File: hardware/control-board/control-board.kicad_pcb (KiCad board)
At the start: 2 copper layers, 39 x 110 mm, 44 parts, among them J10 Conn_01x09_Socket, J11 Conn_01x09_Socket, J12 Conn_01x12_Pin, J9 Conn_01x13_Socket

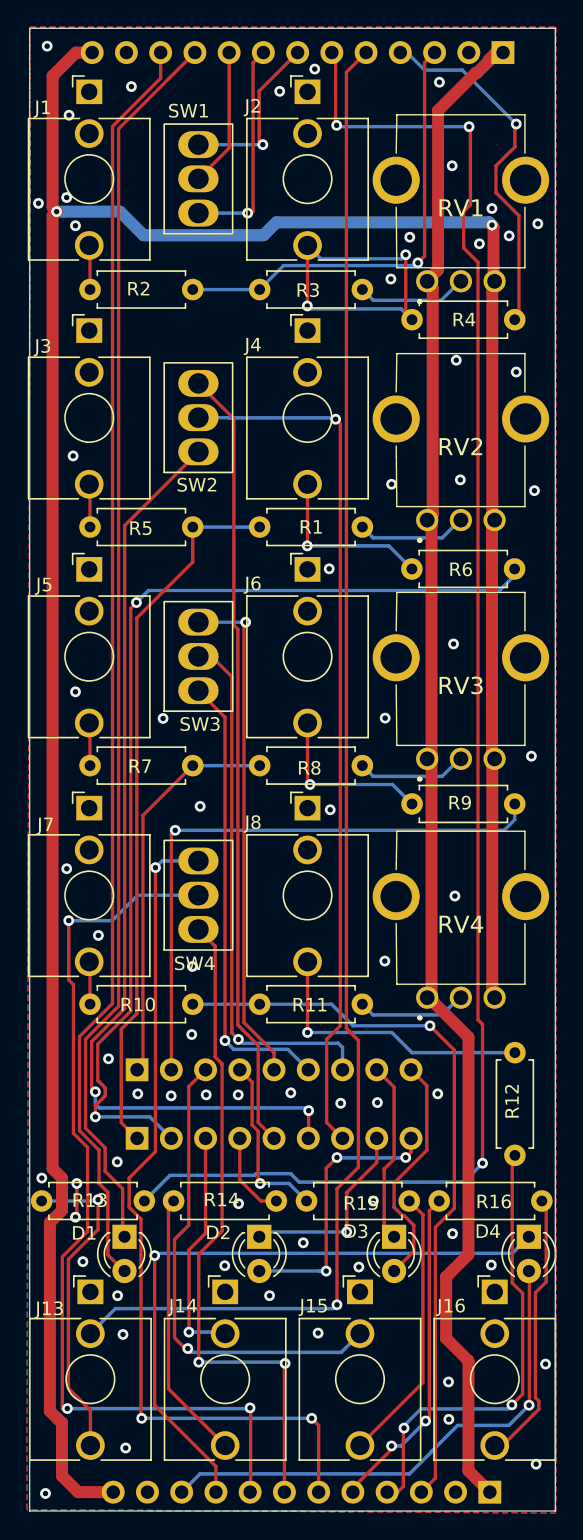
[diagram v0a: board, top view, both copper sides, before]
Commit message: wip - first pass done
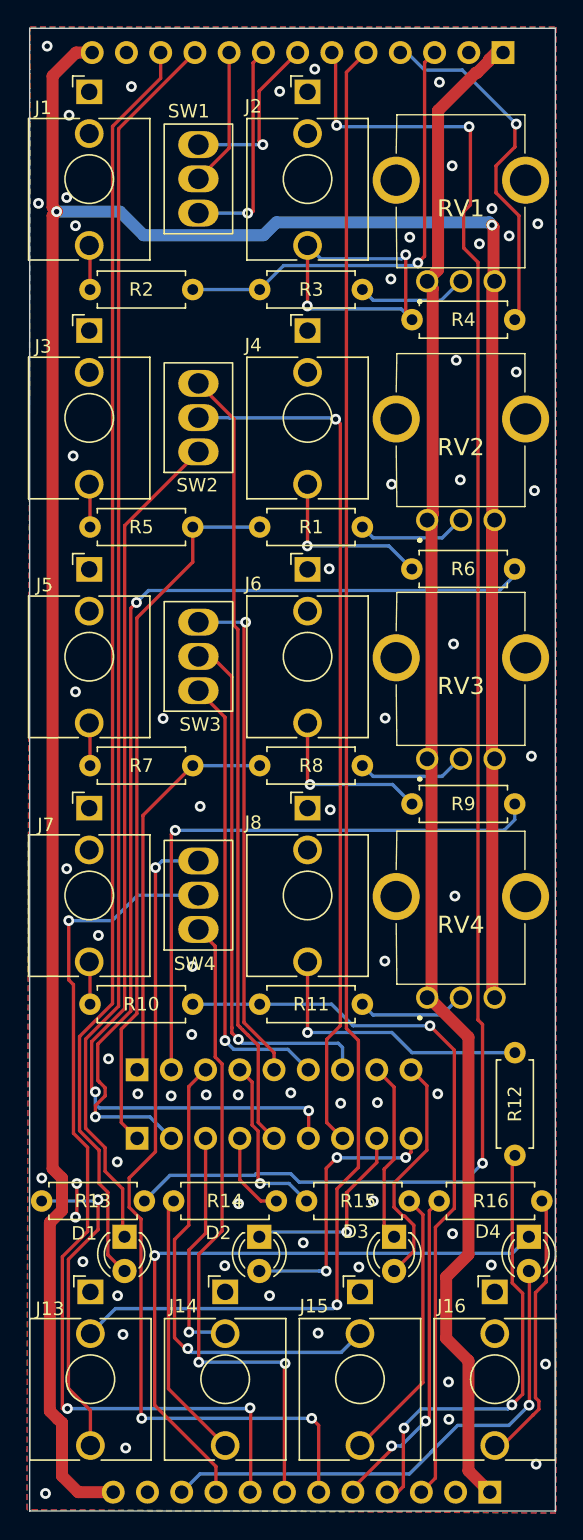
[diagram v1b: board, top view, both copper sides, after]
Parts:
- D1, D2, D3, D4: footprint LED_THT:LED_D3.0mm -> Eurorack Common:LED_D3.0mm
- R1, R10, R11, R12, R13, R14, R15, R16, R2, R3, R4, R5, R6, R7, R8, R9: footprint Resistor_THT:R_Axial_DIN0207_L6.3mm_D2.5mm_P7.62mm_Horizontal -> Eurorack Common:R_Axial_DIN0207_L6.3mm_D2.5mm_P7.62mm_Horizontal
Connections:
- net Net-(J13-PadT) renamed /AUDIO_OUT_A
- net Net-(J14-PadT) renamed /AUDIO_OUT_B
- net Net-(J15-PadT) renamed /AUDIO_OUT_C
- net Net-(J16-PadT) renamed /AUDIO_OUT_MIX
- net Net-(J2-PadT) renamed /AUDIO_IN_A
- net Net-(J4-PadT) renamed /AUDIO_IN_B
- net Net-(J6-PadT) renamed /AUDIO_IN_C
- net Net-(J8-PadT) renamed /AUDIO_IN_D

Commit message: chore: clean up the boards
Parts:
- D1, D2, D3, D4: value LED_Dual_Bidirectional -> Bipolar LED
- J1, J13, J14, J15, J16, J2, J3, J4, J5, J6, J7, J8: value ~ -> Thonkicon
- J10, J11: value Conn_01x09_Socket -> 01x09 Female Pin Header
- J12: value Conn_01x12_Pin -> 01x12 Female Pin Header
- J9: value Conn_01x13_Socket -> 01x13 Female Pin Header
- RV1, RV2, RV3, RV4: value 100K -> A100K
- SW1, SW2, SW3, SW4: value ~ -> Subminiture SPDT
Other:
- board text added: "J2"
